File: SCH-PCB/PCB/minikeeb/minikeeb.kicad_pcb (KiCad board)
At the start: 2 copper layers, 99.8 x 91 mm, 91 parts, among them J1 OLED, SW1 SW_PUSH-Lily58-cache, SW10 SW_PUSH-Lily58-cache, SW11 SW_PUSH-Lily58-cache, SW12 SW_PUSH-Lily58-cache, SW13 SW_PUSH-Lily58-cache, SW14 SW_PUSH-Lily58-cache, SW15 SW_PUSH-Lily58-cache, SW16 SW_PUSH-Lily58-cache, SW17 SW_PUSH-Lily58-cache, SW18 SW_PUSH-Lily58-cache, SW19 SW_PUSH-Lily58-cache, SW2 SW_PUSH-Lily58-cache, SW20 Rotary_Encoder_Switch-Device, SW3 SW_PUSH-Lily58-cache, SW4 SW_PUSH-Lily58-cache, SW5 SW_PUSH-Lily58-cache, SW6 SW_PUSH-Lily58-cache, SW7 SW_PUSH-Lily58-cache, SW8 SW_PUSH-Lily58-cache, SW9 SW_PUSH-Lily58-cache, U1 ProMicro_2-Lily58-cache, U2 TRRS

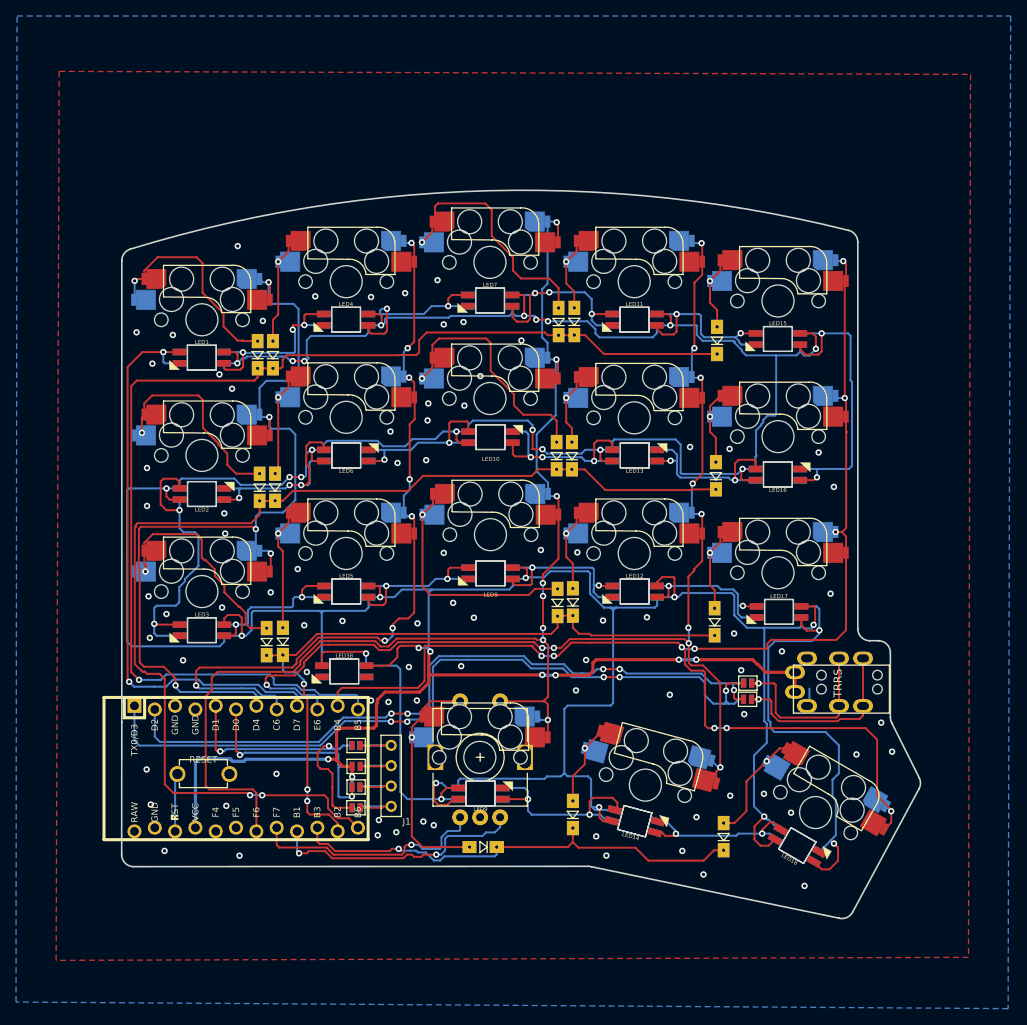
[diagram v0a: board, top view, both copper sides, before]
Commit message: FEAT: add logo and name
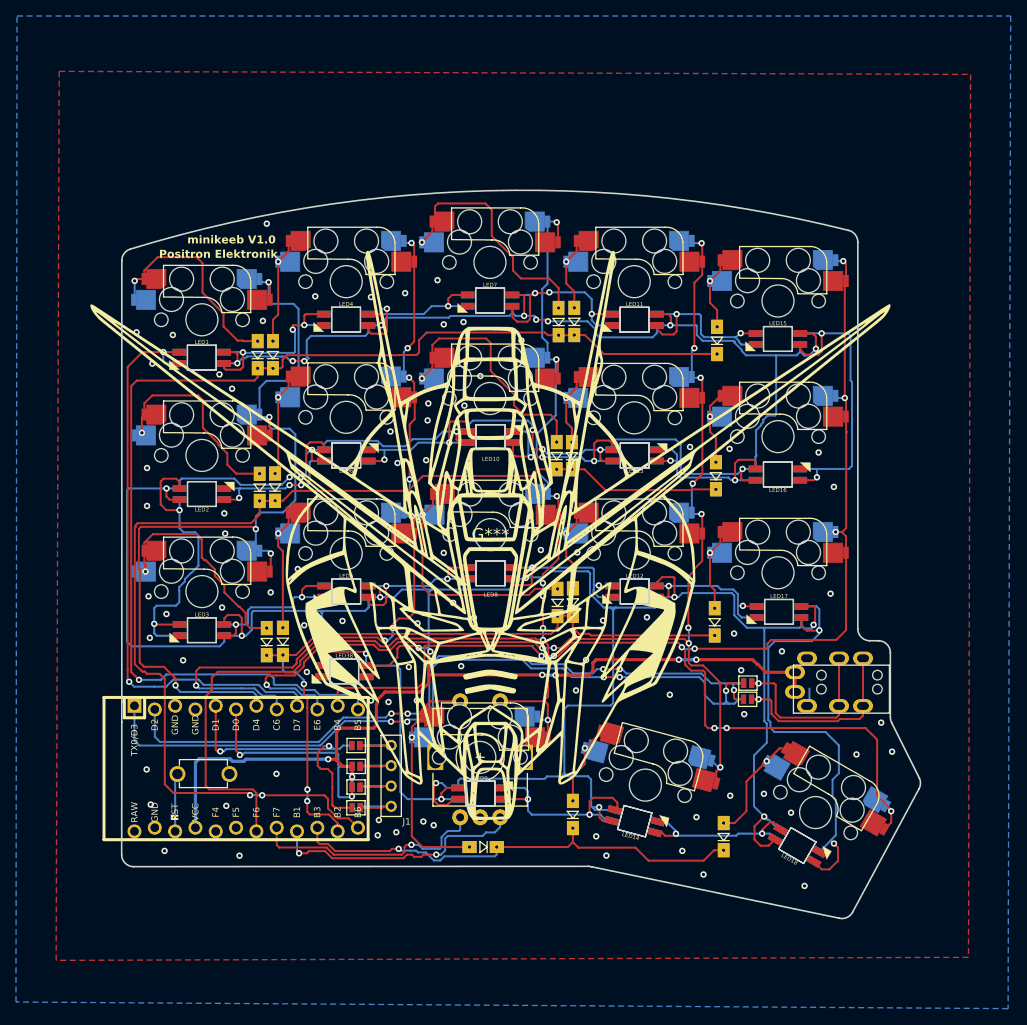
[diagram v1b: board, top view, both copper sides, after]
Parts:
- added G***: LOGO, gundam:gundam, F.Cu at (76.2, 110.0)
- added G***: LOGO, gundam:gundam, B.Cu at (76.2, 110.0)
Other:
- board text added: "Positron Elektronik"
- board text added: "minikeeb V1.0"
